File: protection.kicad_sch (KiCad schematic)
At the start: 33 parts, among them U21 LM339

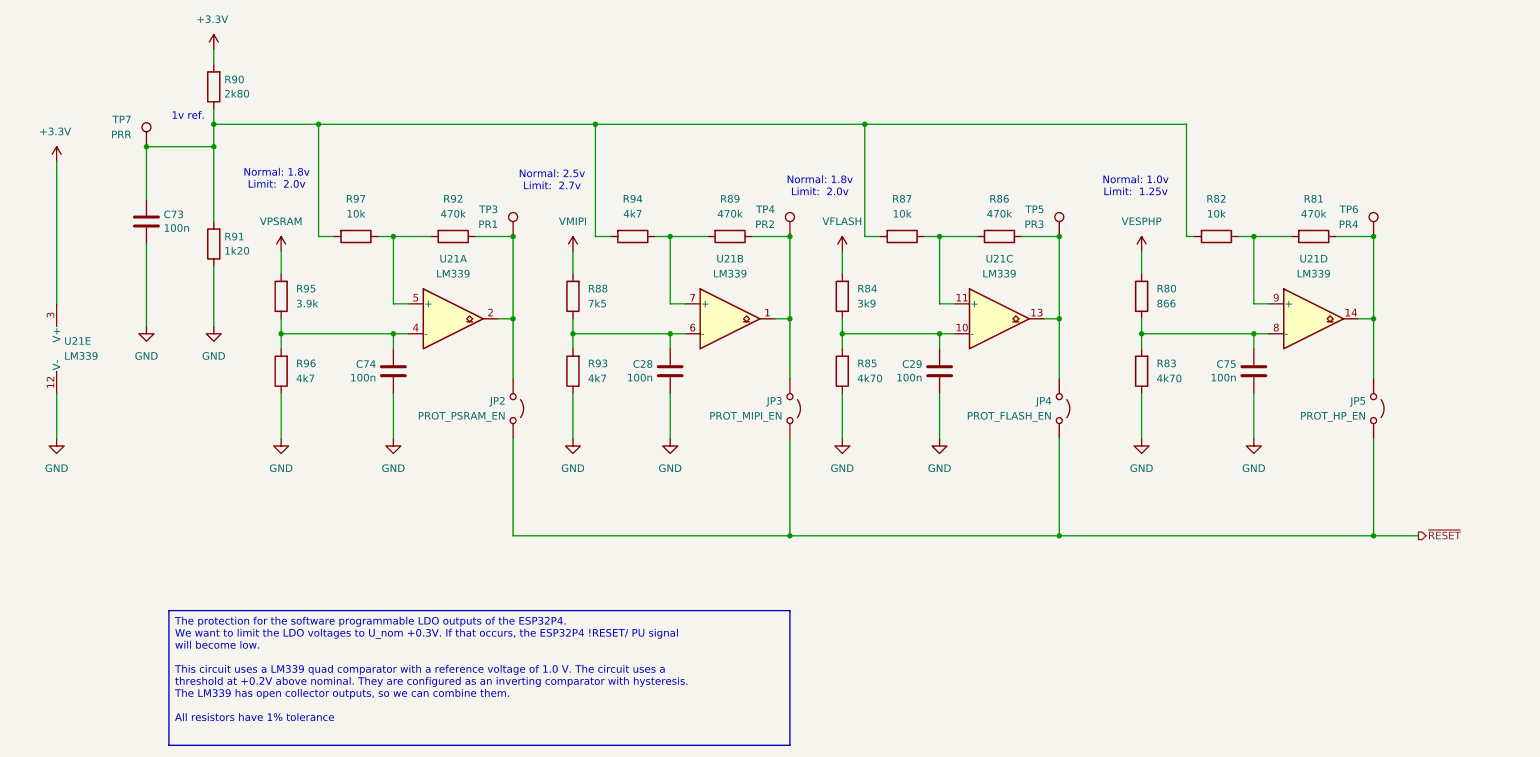
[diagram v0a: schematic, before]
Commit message: Small tweaks and fixes, update LCSC numbers on some components, change to new key type for power key
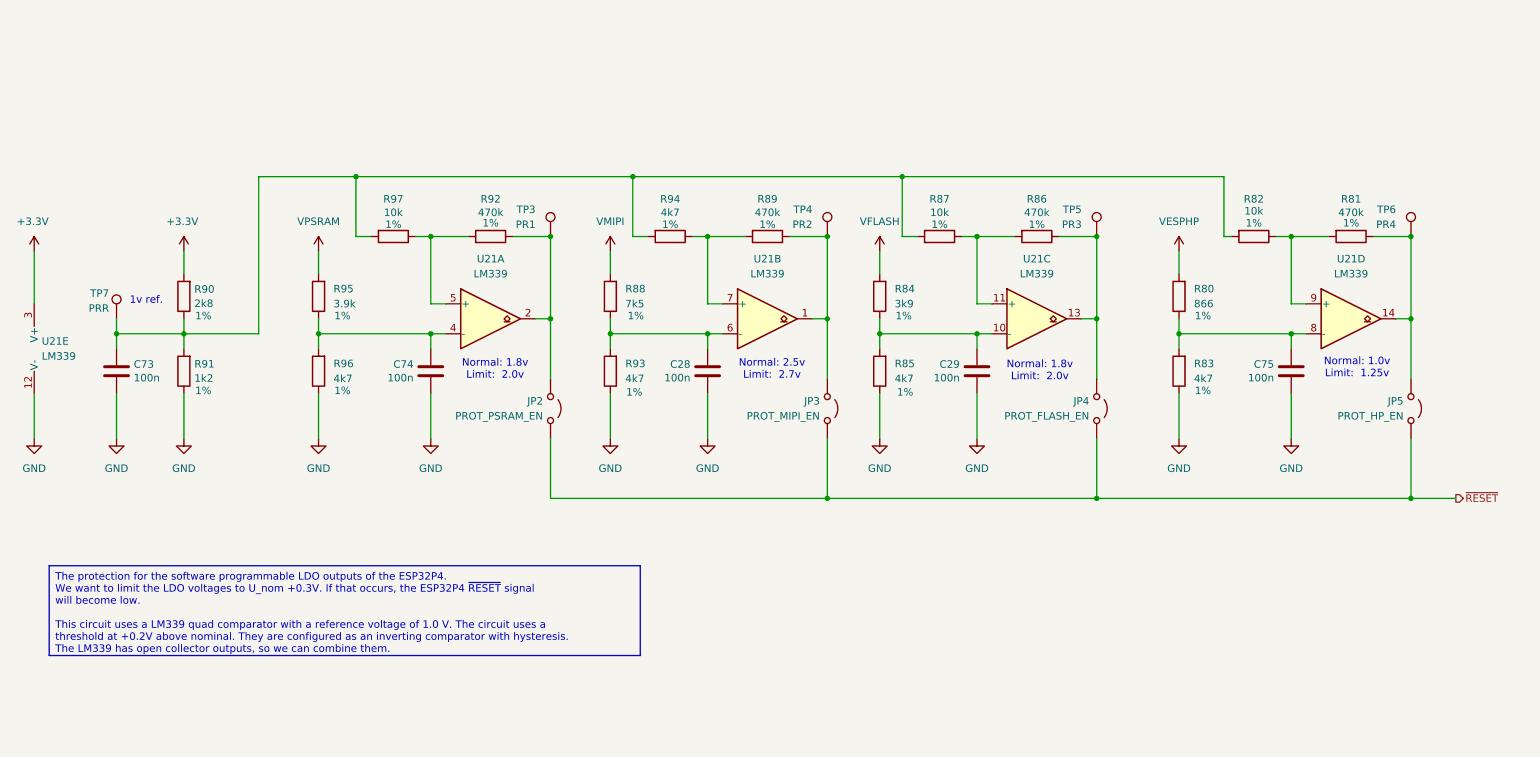
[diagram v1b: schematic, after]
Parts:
- R80: LCSC (none) -> C423129
- R81, R86, R89, R92: LCSC (none) -> C25790
- R83: value 4k70 -> 4k7; LCSC (none) -> C25900
- R84, R95: LCSC C25741 -> C51721
- R85: value 4k70 -> 4k7; LCSC C25741 -> C25900
- R88: LCSC (none) -> C25918
- R90: value 2k80 -> 2k8; LCSC (none) -> C62741
- R91: value 1k20 -> 1k2; LCSC (none) -> C11702
- R93: LCSC (none) -> C25900
- R94: LCSC C60490 -> C25900
- R96: LCSC C25741 -> C25900
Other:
- moved on the sheet: C28, C29, C73, C74, C75, JP2, JP3, JP4, JP5, R80, R81, R82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
